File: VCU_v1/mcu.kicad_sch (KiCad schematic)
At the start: 16 parts, among them SW1 SW_Push, U3 STM32H723ZGT6, Y1 16 MHz, Y2 32.768 kHz

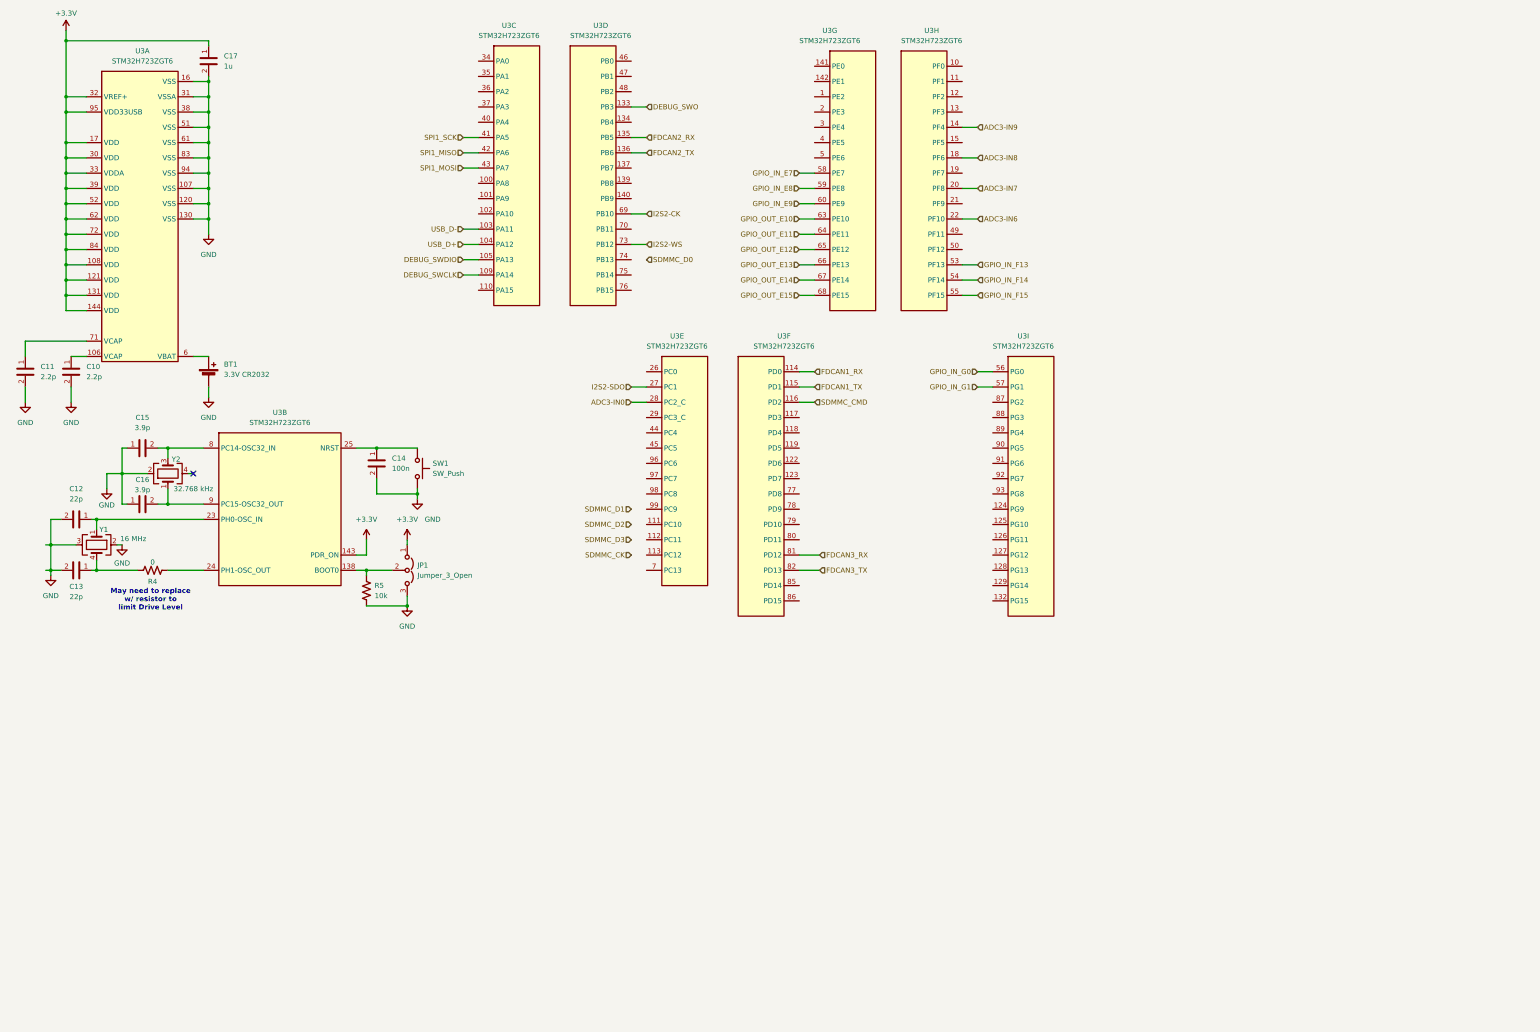
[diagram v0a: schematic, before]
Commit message: left to do before layout: wire DRS/Debug LEDs to connector, add BRUHbus ports
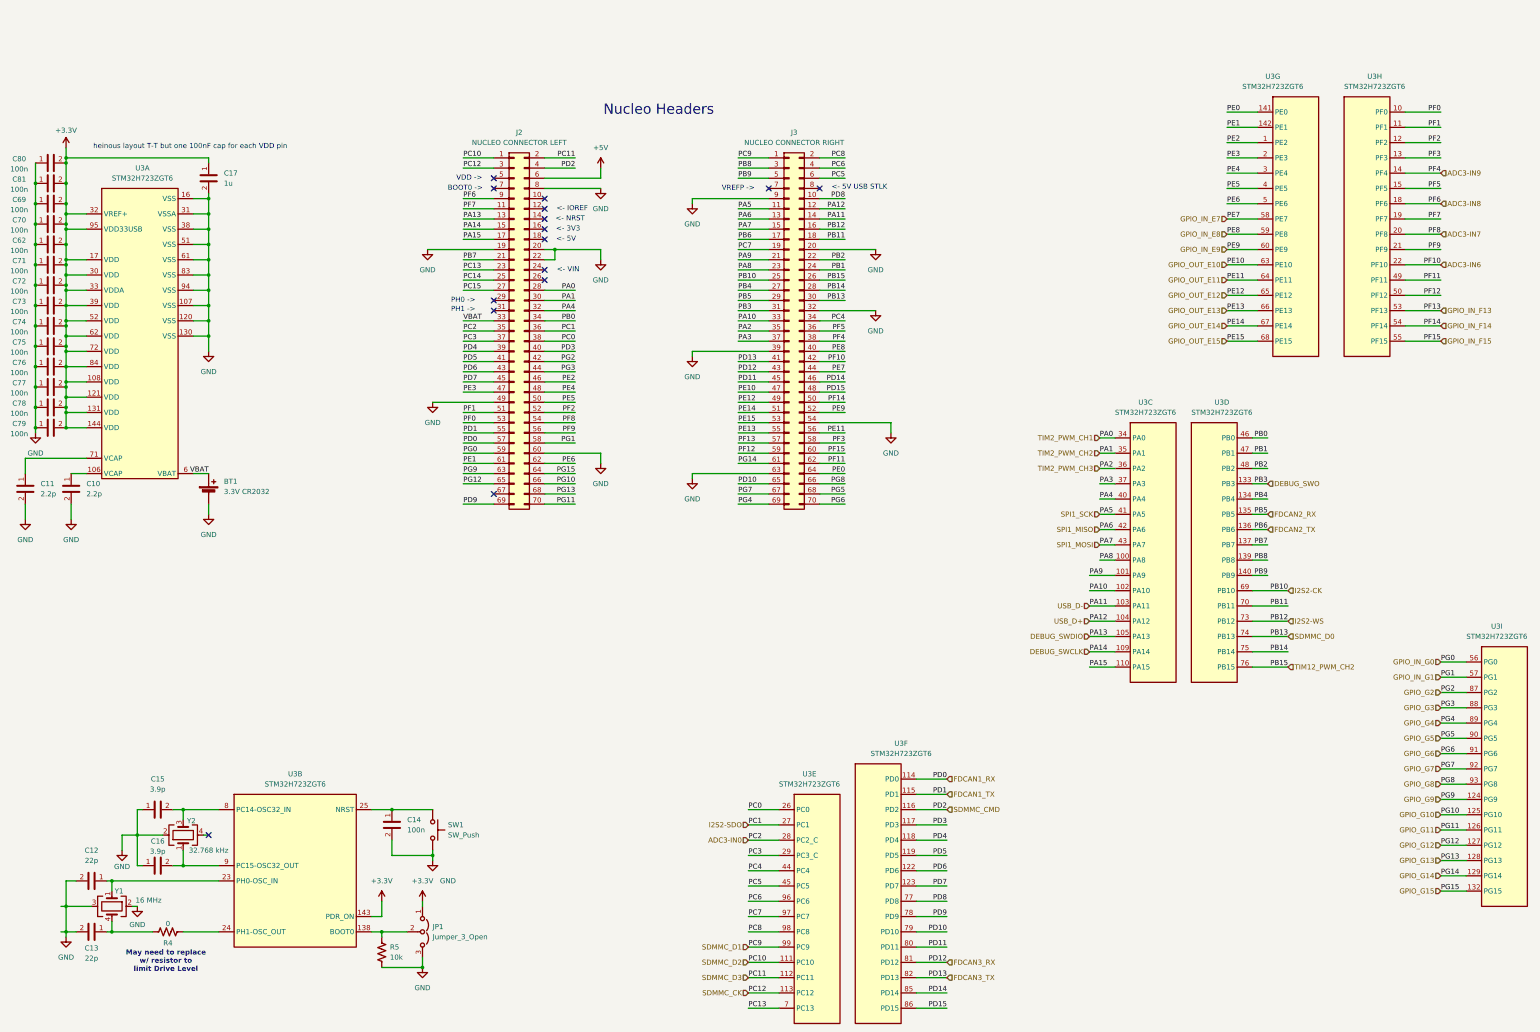
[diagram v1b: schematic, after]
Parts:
- added C62, C69, C70, C71, C72, C73, C74, C75, C76, C77, C78, C79, C80, C81: 100n, Capacitor_SMD:C_0603_1608Metric_Pad1.08x0.95mm_HandSolder, symbol BFR Capacitors:06035C104KAT2A
- added J2: NUCLEO CONNECTOR LEFT, symbol Connector_Generic:Conn_02x35_Odd_Even
- added J3: NUCLEO CONNECTOR RIGHT, symbol Connector_Generic:Conn_02x35_Odd_Even
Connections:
- net +3.3V: now also C62.2, C69.2, C70.2, C71.2, C72.2, C73.2, C74.2, C75.2, C76.2, C77.2, C78.2, C79.2, C80.2, C81.2
- net ADC3-IN0: now also J2.35 (Pin_35)
- net ADC3-IN6: now also J3.42 (Pin_42)
- net ADC3-IN7: now also J2.54 (Pin_54)
- net ADC3-IN8: now also J2.9 (Pin_9)
- net ADC3-IN9: now also J3.38 (Pin_38)
- net DEBUG_SWCLK: now also J2.15 (Pin_15)
- net DEBUG_SWDIO: now also J2.13 (Pin_13)
- net DEBUG_SWO: now also J3.31 (Pin_31)
- net FDCAN1_RX: now also J2.57 (Pin_57)
- net FDCAN1_TX: now also J2.55 (Pin_55)
- net FDCAN2_RX: now also J3.29 (Pin_29)
- net FDCAN2_TX: now also J3.17 (Pin_17)
- net FDCAN3_RX: now also J3.43 (Pin_43)
- net FDCAN3_TX: now also J3.41 (Pin_41)
- net GND: now also C62.1, C69.1, C70.1, C71.1, C72.1, C73.1, C74.1, C75.1, C76.1, C77.1, C78.1, C79.1, C80.1, C81.1, J2.19 (Pin_19), J2.20 (Pin_20), J2.22 (Pin_22), J2.49 (Pin_49), J2.60 (Pin_60), J2.8 (Pin_8), J3.20 (Pin_20), J3.32 (Pin_32), J3.39 (Pin_39), J3.54 (Pin_54), J3.63 (Pin_63), J3.9 (Pin_9)
- net GPIO_IN_E7: now also J3.44 (Pin_44)
- net GPIO_IN_E8: now also J3.40 (Pin_40)
- net GPIO_IN_E9: now also J3.52 (Pin_52)
- net GPIO_IN_F13: now also J3.57 (Pin_57)
- net GPIO_IN_F14: now also J3.50 (Pin_50)
- net GPIO_IN_F15: now also J3.60 (Pin_60)
- net GPIO_IN_G0: now also J2.59 (Pin_59)
- net GPIO_IN_G1: now also J2.58 (Pin_58)
- net GPIO_OUT_E10: now also J3.47 (Pin_47)
- net GPIO_OUT_E11: now also J3.56 (Pin_56)
- net GPIO_OUT_E12: now also J3.49 (Pin_49)
- net GPIO_OUT_E13: now also J3.55 (Pin_55)
- net GPIO_OUT_E14: now also J3.51 (Pin_51)
- net GPIO_OUT_E15: now also J3.53 (Pin_53)
- net I2S2-CK: now also J3.25 (Pin_25)
- net I2S2-SDO: now also J2.36 (Pin_36)
- net I2S2-WS: now also J3.16 (Pin_16)
- net SDMMC_CK: now also U3.113 (PC12), J2.3 (Pin_3)
- net SDMMC_CMD: now also J2.4 (Pin_4)
- net SDMMC_D0: now also U3.74 (PB13), J3.30 (Pin_30)
- net SDMMC_D1: now also U3.99 (PC9), J3.1 (Pin_1)
- net SDMMC_D2: now also U3.111 (PC10), J2.1 (Pin_1)
- net SDMMC_D3: now also U3.112 (PC11), J2.2 (Pin_2)
- net SPI1_MISO: now also J3.13 (Pin_13)
- net SPI1_MOSI: now also J3.15 (Pin_15)
- net SPI1_SCK: now also J3.11 (Pin_11)
- net USB_D+: now also J3.12 (Pin_12)
- net USB_D-: now also J3.14 (Pin_14)
- net PA8: now reaches U3.100 (PA8)
- net PA8: now also J3.23 (Pin_23)
- net PA9: now reaches U3.101 (PA9)
- net PA9: now also J3.21 (Pin_21)
- net PA10: now reaches U3.102 (PA10)
- net PA10: now also J3.33 (Pin_33)
- net PA15: now reaches U3.110 (PA15)
- net PA15: now also J2.17 (Pin_17)
- net TIM2_PWM_CH1: now reaches U3.34 (PA0)
- net TIM2_PWM_CH1: now also J2.28 (Pin_28)
- net TIM2_PWM_CH2: now reaches U3.35 (PA1)
- net TIM2_PWM_CH2: now also J2.30 (Pin_30)
- net TIM2_PWM_CH3: now reaches U3.36 (PA2)
- net TIM2_PWM_CH3: now also J3.35 (Pin_35)
- net PA3: now reaches U3.37 (PA3)
- net PA3: now also J3.37 (Pin_37)
- net PA4: now reaches U3.40 (PA4)
- net PA4: now also J2.32 (Pin_32)
- net PD3: now reaches U3.117 (PD3)
- net PD3: now also J2.40 (Pin_40)
- net PD4: now reaches U3.118 (PD4)
- net PD4: now also J2.39 (Pin_39)
- net PD5: now reaches U3.119 (PD5)
- net PD5: now also J2.41 (Pin_41)
- net PD6: now reaches U3.122 (PD6)
- net PD6: now also J2.43 (Pin_43)
- net PD7: now reaches U3.123 (PD7)
- net PD7: now also J2.45 (Pin_45)
- net PD8: now reaches U3.77 (PD8)
- net PD8: now also J3.10 (Pin_10)
- net PD9: now reaches U3.78 (PD9)
- net PD9: now also J2.69 (Pin_69)
- net PD10: now reaches U3.79 (PD10)
- net PD10: now also J3.65 (Pin_65)
- net PD11: now reaches U3.80 (PD11)
- net PD11: now also J3.45 (Pin_45)
- net PD14: now reaches U3.85 (PD14)
- net PD14: now also J3.46 (Pin_46)
- net PD15: now reaches U3.86 (PD15)
- net PD15: now also J3.48 (Pin_48)
- net PE2: now reaches U3.1 (PE2)
- net PE2: now also J2.46 (Pin_46)
- net PE0: now reaches U3.141 (PE0)
- net PE0: now also J3.64 (Pin_64)
- net PE1: now reaches U3.142 (PE1)
- net PE1: now also J2.61 (Pin_61)
- net PE3: now reaches U3.2 (PE3)
- net PE3: now also J2.47 (Pin_47)
- net PE4: now reaches U3.3 (PE4)
- net PE4: now also J2.48 (Pin_48)
- net PE5: now reaches U3.4 (PE5)
- net PE5: now also J2.50 (Pin_50)
- net PE6: now reaches U3.5 (PE6)
- net PE6: now also J2.62 (Pin_62)
- net VBAT: now reaches BT1.1 (+), U3.6 (VBAT)
- net VBAT: now also J2.33 (Pin_33)
- net PF0: now reaches U3.10 (PF0)
- net PF0: now also J2.53 (Pin_53)
- net PF1: now reaches U3.11 (PF1)
- net PF1: now also J2.51 (Pin_51)
- net PF2: now reaches U3.12 (PF2)
- net PF2: now also J2.52 (Pin_52)
- net PF3: now reaches U3.13 (PF3)
- net PF3: now also J3.58 (Pin_58)
- net PF5: now reaches U3.15 (PF5)
- net PF5: now also J3.36 (Pin_36)
- net PF7: now reaches U3.19 (PF7)
- net PF7: now also J2.11 (Pin_11)
- net PF9: now reaches U3.21 (PF9)
- net PF9: now also J2.56 (Pin_56)
- net PF11: now reaches U3.49 (PF11)
- net PF11: now also J3.62 (Pin_62)
- net PF12: now reaches U3.50 (PF12)
- net PF12: now also J3.59 (Pin_59)
- net PC0: now reaches U3.26 (PC0)
- net PC0: now also J2.38 (Pin_38)
- net PC3: now reaches U3.29 (PC3_C)
- net PC3: now also J2.37 (Pin_37)
- net PC4: now reaches U3.44 (PC4)
- net PC4: now also J3.34 (Pin_34)
- net PC5: now reaches U3.45 (PC5)
- net PC5: now also J3.6 (Pin_6)
- net PC13: now reaches U3.7 (PC13)
- net PC13: now also J2.23 (Pin_23)
- net PC6: now reaches U3.96 (PC6)
- net PC6: now also J3.4 (Pin_4)
- net PC7: now reaches U3.97 (PC7)
- net PC7: now also J3.19 (Pin_19)
- net PC8: now reaches U3.98 (PC8)
- net PC8: now also J3.2 (Pin_2)
- net PB4: now reaches U3.134 (PB4)
- net PB4: now also J3.27 (Pin_27)
- net PB7: now reaches U3.137 (PB7)
- net PB7: now also J2.21 (Pin_21)
- net PB8: now reaches U3.139 (PB8)
- net PB8: now also J3.3 (Pin_3)
- net PB9: now reaches U3.140 (PB9)
- net PB9: now also J3.5 (Pin_5)
- net PB0: now reaches U3.46 (PB0)
- net PB0: now also J2.34 (Pin_34)
- net PB1: now reaches U3.47 (PB1)
- net PB1: now also J3.24 (Pin_24)
- net PB2: now reaches U3.48 (PB2)
- net PB2: now also J3.22 (Pin_22)
- net PB11: now reaches U3.70 (PB11)
- net PB11: now also J3.18 (Pin_18)
- net PB14: now reaches U3.75 (PB14)
- net PB14: now also J3.28 (Pin_28)
- net TIM12_PWM_CH2: now reaches U3.76 (PB15)
- net TIM12_PWM_CH2: now also J3.26 (Pin_26)
- net GPIO_G9: now reaches U3.124 (PG9)
- net GPIO_G9: now also J2.63 (Pin_63)
- net GPIO_G10: now reaches U3.125 (PG10)
- net GPIO_G10: now also J2.66 (Pin_66)
- net GPIO_G11: now reaches U3.126 (PG11)
- net GPIO_G11: now also J2.70 (Pin_70)
- net GPIO_G12: now reaches U3.127 (PG12)
- net GPIO_G12: now also J2.65 (Pin_65)
- net GPIO_G13: now reaches U3.128 (PG13)
- net GPIO_G13: now also J2.68 (Pin_68)
- net GPIO_G14: now reaches U3.129 (PG14)
- net GPIO_G14: now also J3.61 (Pin_61)
- net GPIO_G15: now reaches U3.132 (PG15)
- net GPIO_G15: now also J2.64 (Pin_64)
- net GPIO_G2: now reaches U3.87 (PG2)
- net GPIO_G2: now also J2.42 (Pin_42)
- net GPIO_G3: now reaches U3.88 (PG3)
- net GPIO_G3: now also J2.44 (Pin_44)
- net GPIO_G4: now reaches U3.89 (PG4)
- net GPIO_G4: now also J3.69 (Pin_69)
- net GPIO_G5: now reaches U3.90 (PG5)
- net GPIO_G5: now also J3.68 (Pin_68)
- net GPIO_G6: now reaches U3.91 (PG6)
- net GPIO_G6: now also J3.70 (Pin_70)
- net GPIO_G7: now reaches U3.92 (PG7)
- net GPIO_G7: now also J3.67 (Pin_67)
- net GPIO_G8: now reaches U3.93 (PG8)
- net GPIO_G8: now also J3.66 (Pin_66)
- new net +5V: J2.6 (Pin_6)
- new net PC14: J2.25 (Pin_25)
- new net PC15: J2.27 (Pin_27)
- no-connect marks 1 -> 15
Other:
- note added: "<- 3V3"
- note added: "<- 5V"
- note added: "<- 5V USB STLK"
- note added: "<- IOREF"
- note added: "<- NRST"
- note added: "<- VIN"
- note added: "BOOT0 ->"
- note added: "Nucleo Headers"
- note added: "PH0 ->"
- note added: "PH1 ->"
- note added: "VDD ->"
- note added: "VREFP ->"
- note added: "heinous layout T-T but one 100nF cap for each VDD pin"
- moved on the sheet: BT1, C10, C11, C12, C13, C14, C15, C16, C17, JP1, R4, R5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
